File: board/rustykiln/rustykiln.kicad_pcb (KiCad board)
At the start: 2 copper layers, 14 parts, among them IC1 TPS5450DDA, J1 MPM-15-24, U1 RP2040_Stamp

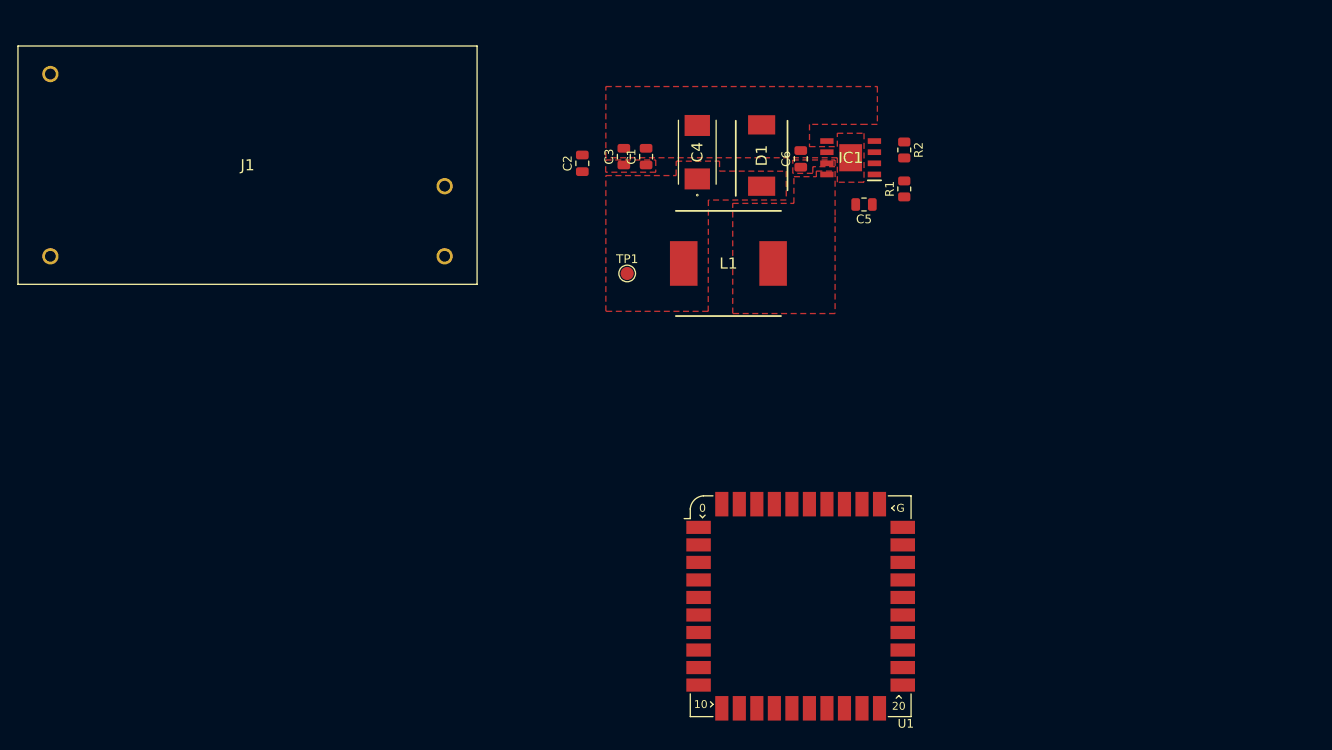
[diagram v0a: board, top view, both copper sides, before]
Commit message: Updates
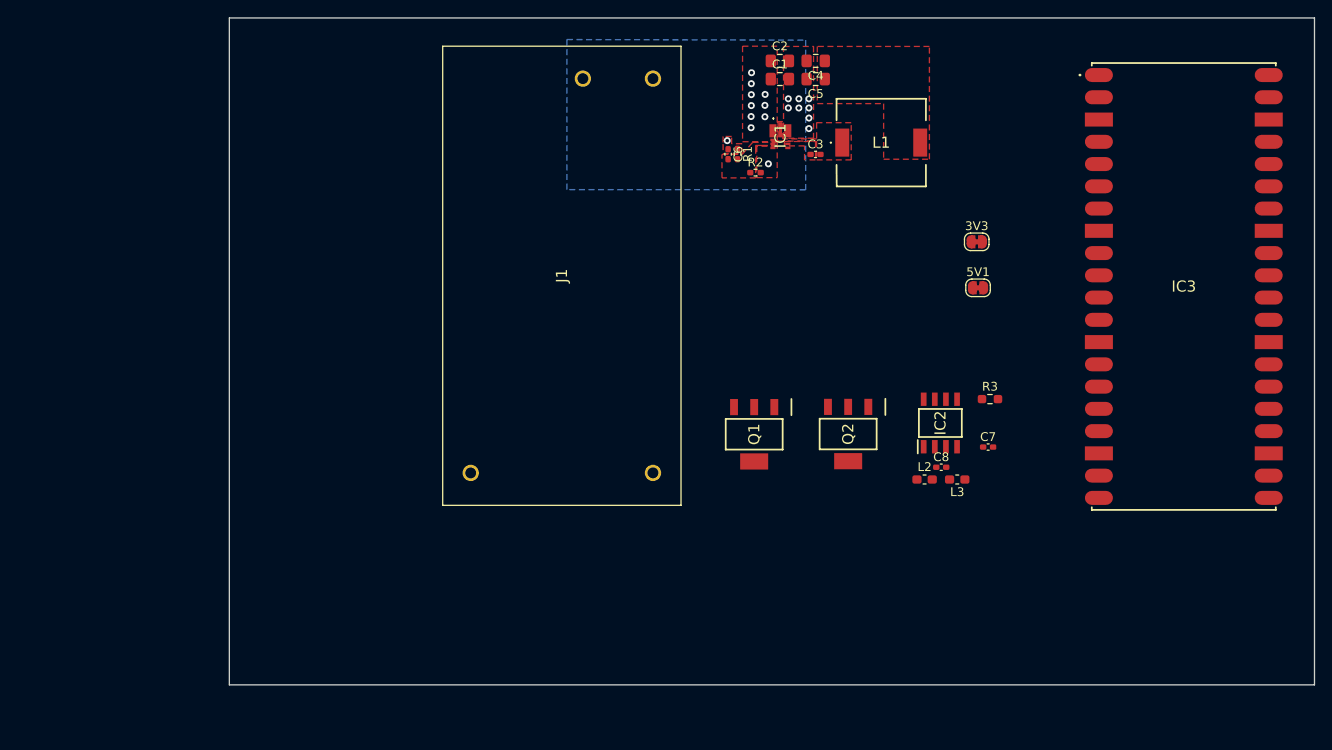
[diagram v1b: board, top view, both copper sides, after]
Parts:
- removed D1: B540C, SamacSys_Parts:DIOM7959X250N
- removed TP1: 5V, TestPoint:TestPoint_Pad_D1.5mm
- removed U1: RP2040_Stamp, RP2040:RP2040_Stamp_SMD
- added 3V3: SolderJumper_2_Bridged, Jumper:SolderJumper-2_P1.3mm_Bridged_RoundedPad1.0x1.5mm, F.Cu at (165.5, 87.5)
- added 5V1: SolderJumper_2_Bridged, Jumper:SolderJumper-2_P1.3mm_Bridged_RoundedPad1.0x1.5mm, F.Cu at (165.7, 92.8)
- added C7: 0.1uF, Capacitor_SMD:C_0402_1005Metric_Pad0.74x0.62mm_HandSolder, F.Cu at (166.8, 111.0)
- added C8: 10nF, Capacitor_SMD:C_0402_1005Metric_Pad0.74x0.62mm_HandSolder, F.Cu at (161.5, 113.3)
- added IC2: MAX31855KASA+T, libs:SOIC127P600X175-8N, F.Cu at (161.4, 108.2)
- added IC3: RASPBERRY_PI_PICO_W, libs:RASPBERRYPIPICOW, F.Cu at (189.2, 92.6)
- added L2: 470Ohm, Inductor_SMD:L_0603_1608Metric_Pad1.05x0.95mm_HandSolder, F.Cu at (159.6, 114.7)
- added L3: 470Ohm, Inductor_SMD:L_0603_1608Metric_Pad1.05x0.95mm_HandSolder, F.Cu at (163.3, 114.7)
- added Q1: ZXMS6006SGTA, libs:SOT230P700X170-4N, F.Cu at (140.1, 109.5)
- added Q2: ZXMS6006SGTA, libs:SOT230P700X170-4N, F.Cu at (150.8, 109.5)
- added R3: 10k, Resistor_SMD:R_0603_1608Metric_Pad0.98x0.95mm_HandSolder, F.Cu at (167.0, 105.5)
- C1: footprint Capacitor_SMD:C_0805_2012Metric -> Capacitor_SMD:C_0805_2012Metric_Pad1.18x1.45mm_HandSolder
- C2: value 0.01uF -> 4.7uF; footprint Capacitor_SMD:C_0805_2012Metric -> Capacitor_SMD:C_0805_2012Metric_Pad1.18x1.45mm_HandSolder
- C3: value 4.7uF -> 0.1uF; footprint Capacitor_SMD:C_0805_2012Metric -> Capacitor_SMD:C_0402_1005Metric_Pad0.74x0.62mm_HandSolder
- C4: value 330uF -> 22uF; footprint SamacSys_Parts:POSCAP_D12_D15_D15E_D2E_D2_D3L_D4 -> Capacitor_SMD:C_0805_2012Metric_Pad1.18x1.45mm_HandSolder
- C5: value 0.01uF -> 22uF; footprint Capacitor_SMD:C_0805_2012Metric -> Capacitor_SMD:C_0805_2012Metric_Pad1.18x1.45mm_HandSolder
- C6: value 0.01uF -> 47pF; footprint Capacitor_SMD:C_0805_2012Metric -> Capacitor_SMD:C_0402_1005Metric_Pad0.74x0.62mm_HandSolder
- IC1: value TPS5450DDA -> AP63357DV-7; footprint SamacSys_Parts:SOIC127P600X170-9N -> libs:AP63357DV7
- J1: footprint SamacSys_Parts:MPM1524 -> libs:MPM1524
- L1: value 15uH -> 6.8uH; footprint SamacSys_Parts:INDPM120120X800N -> libs:CDRH103RNP6R8NCB
- R1: value 3.16k -> 220K; footprint Resistor_SMD:R_0805_2012Metric -> Resistor_SMD:R_0402_1005Metric_Pad0.72x0.64mm_HandSolder
- R2: value 10k -> 41.2K; footprint Resistor_SMD:R_0805_2012Metric -> Resistor_SMD:R_0402_1005Metric_Pad0.72x0.64mm_HandSolder
- moved C2 25.4 mm to (143.1, 66.9), turned to 0 degrees
- moved L1 22.2 mm to (154.6, 76.2), turned to 0 degrees
- moved C3 21.9 mm to (147.1, 77.6), turned to 0 degrees
- moved J1 20.0 mm to (120.6, 68.9), turned to -90 degrees
- moved R1 19.4 mm to (138.2, 77.5), turned to -90 degrees
- moved C1 17.7 mm to (143.1, 69.0), turned to 0 degrees
- moved R2 17.2 mm to (140.3, 79.7), turned to 0 degrees
- moved C4 17.1 mm to (147.2, 66.9), turned to 180 degrees
- moved C5 15.3 mm to (147.2, 69.0)
- moved IC1 8.38 mm to (143.1, 75.5), turned to -90 degrees
- moved C6 8.31 mm to (137.2, 77.5), turned to -90 degrees
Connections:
- C2 pad 1: 5V -> 24V
- C3 pad 1: 24V -> /Power/BST
- C3 pad 2: GND -> /Power/SW
- C5 pad 1: Net-(C5-Pad1) -> 5V
- C5 pad 2: /5Vunf -> GND
- C6 pad 1: 24V -> 5V
- C6 pad 2: GND -> /Power/FB
- IC1 pad 1: Net-(C5-Pad1) -> 24V
- IC1 pad 2: unconnected-(IC1-Pad2) -> 24V
- IC1 pad 3: unconnected-(IC1-Pad3) -> /Power/FB
- IC1 pad 4: Net-(IC1-Pad4) -> GND
- IC1 pad 6: GND -> /Power/BST
- IC1 pad 8: /5Vunf -> GND
- IC1 pad 9: GND -> /Power/SW
- L1 pad 1: /5Vunf -> /Power/SW
- R1 pad 1: GND -> 5V
- R1 pad 2: Net-(IC1-Pad4) -> /Power/FB
- R2 pad 1: Net-(IC1-Pad4) -> /Power/FB
- R2 pad 2: 5V -> GND
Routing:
- net GND: vias 0 -> 9
- net 5V: vias 0 -> 1
- net 24V: vias 0 -> 9
- added copper zone on F.Cu, net /Power/BST
- added copper zone on F.Cu, net /Power/FB
- added copper zone on F.Cu, net /Power/SW
- added copper zone on B.Cu, net 24V
- added copper zone on In1.Cu, net GND
- added copper zone on In2.Cu, net GND
- removed copper zone on F.Cu, net /5Vunf
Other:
- board outline added: 123.8 x 76.1 mm
- copper layers 2 -> 4
